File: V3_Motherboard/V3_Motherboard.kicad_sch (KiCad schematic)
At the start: 62 parts, among them J1 Conn_01x16_Pin, J10 Conn_02x04_Row_Letter_First, J14_GND2 Conn_01x03, J14_GND3 Conn_01x03, J18_VDC1 Conn_01x02, J2 Conn_01x16_Pin, J3 Conn_01x16_Pin, J4 Conn_01x16_Pin, J5 PINHD_1x2_Male, J6 Conn_01x02_Pin, J7 PINHD_1x2_Male, J8 PINHD_1x2_Male, J9 Conn_02x03_Counter_Clockwise, U1 NCV8164ASN250T1G_LDO_2.5V, U2 LTC4365TS8, U3 UM6K34NTCN

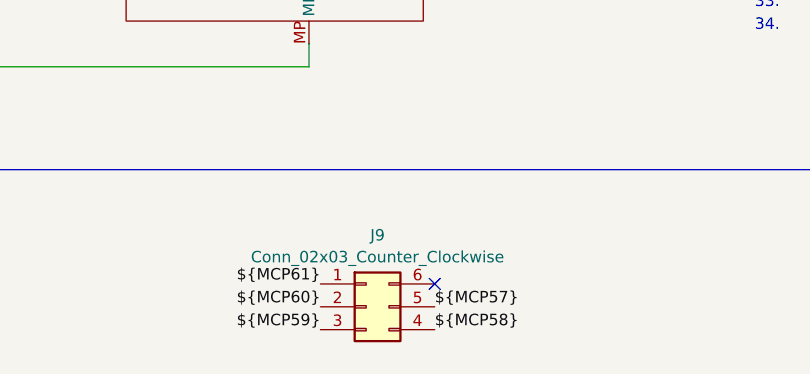
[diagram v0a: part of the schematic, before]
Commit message: Modded
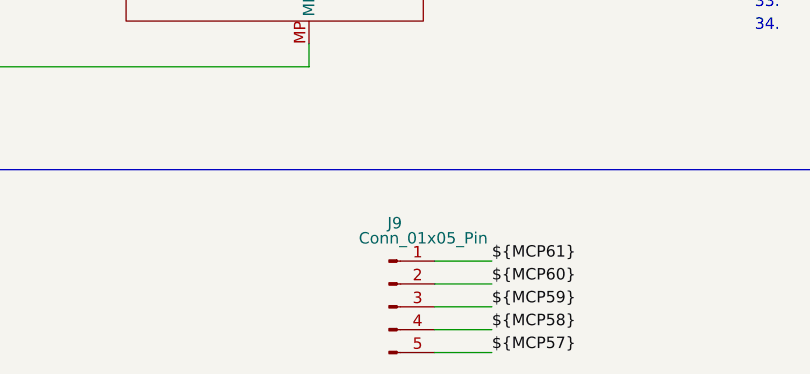
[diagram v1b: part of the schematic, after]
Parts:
- removed J9: Conn_02x03_Counter_Clockwise, Connector_PinHeader_2.54mm:PinHeader_2x03_P2.54mm_Vertical, symbol Connector_Generic:Conn_02x03_Counter_Clockwise
- added J9: Conn_01x05_Pin, Connector_PinHeader_2.54mm:PinHeader_1x05_P2.54mm_Vertical, symbol Connector:Conn_01x05_Pin
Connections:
- net ${MCP57}: now also J9.5 (Pin_5)
- net ${MCP58}: now also J9.4 (Pin_4)
- net ${MCP59}: now also J9.3 (Pin_3)
- net ${MCP60}: now also J9.2 (Pin_2)
- net ${MCP61}: now also J9.1 (Pin_1)
- no-connect marks 8 -> 7
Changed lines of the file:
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@@
 	)
 	(no_connect
-		(at 246.38 264.16)
-	)
-	(no_connect
 		(at 388.62 176.53)
 	)
@@
 	(wire
 		(pts
+			(xy 246.38 271.78) (xy 252.73 271.78)
+		)
+		(stroke
+			(width 0)
+			(type default)
+		)
+	)
+	(wire
+		(pts
 			(xy 318.77 36.83) (xy 316.23 36.83)
 		)
@@
 		)
 	)
+	(wire
+		(pts
+			(xy 246.38 269.24) (xy 252.73 269.24)
+		)
+		(stroke
+			(width 0)
+			(type default)
+		)
+	)
 	(polyline
 		(pts
@@
 	(wire
 		(pts
+			(xy 252.73 261.62) (xy 246.38 261.62)
+		)
+		(stroke
+			(width 0)
+			(type default)
+		)
+	)
+	(wire
+		(pts
 			(xy 317.5 39.37) (xy 328.93 39.37)
 		)
@@
 	(wire
 		(pts
+			(xy 252.73 266.7) (xy 246.38 266.7)
+		)
+		(stroke
+			(width 0)
+			(type default)
+		)
+	)
+	(wire
+		(pts
 			(xy 46.99 99.06) (xy 46.99 113.03)
 		)
@@
 		)
 	)
+	(wire
+		(pts
+			(xy 252.73 264.16) (xy 246.38 264.16)
+		)
+		(stroke
+			(width 0)
+			(type default)
+		)
+	)
 	(polyline
 		(pts
@@
 		)
 	)
-	(label "${MCP61}"
-		(at 233.68 264.16 180)
-		(effects
-			(font
-				(size 1.27 1.27)
-			)
-			(justify right bottom)
-		)
-	)
 	(label "${MCP16}"
 		(at 187.96 170.18 0)
@@
 		)
 	)
+	(label "${MCP59}"
+		(at 252.73 266.7 0)
+		(effects
+			(font
+				(size 1.27 1.27)
+			)
+			(justify left bottom)
+		)
+	)
+	(label "${MCP57}"
+		(at 252.73 271.78 0)
+		(effects
+			(font
+				(size 1.27 1.27)
+			)
+			(justify left bottom)
+		)
+	)
 	(label "${MCP46}"
 		(at 270.51 195.58 180)
@@
 		)
 	)
+	(label "${MCP58}"
+		(at 252.73 269.24 0)
+		(effects
+			(font
+				(size 1.27 1.27)
+			)
+			(justify left bottom)
+		)
+	)
 	(label "${MCP64}"
 		(at 186.69 223.52 0)
@@
 		)
 	)
-	(label "${MCP58}"
-		(at 246.38 269.24 0)
-		(effects
-			(font
-				(size 1.27 1.27)
-			)
-			(justify left bottom)
-		)
-	)
 	(label "${MCP53}"
 		(at 270.51 213.36 180)
@@
 		)
 	)
-	(label "${MCP59}"
-		(at 233.68 269.24 180)
-		(effects
-			(font
-				(size 1.27 1.27)
-			)
-			(justify right bottom)
-		)
-	)
 	(label "${MCP7}"
 		(at 187.96 193.04 0)
@@
 		)
 	)
-	(label "${MCP60}"
-		(at 233.68 266.7 180)
-		(effects
-			(font
-				(size 1.27 1.27)
-			)
-			(justify right bottom)
-		)
-	)
 	(label "VDD"
 		(at 191.77 144.78 180)
@@
 		)
 	)
-	(label "${MCP57}"
-		(at 246.38 266.7 0)
-		(effects
-			(font
-				(size 1.27 1.27)
-			)
-			(justify left bottom)
-		)
-	)
 	(label "${MCP52}"
 		(at 270.51 210.82 180)
@@
 		)
 	)
+	(label "${MCP60}"
+		(at 252.73 264.16 0)
+		(effects
+			(font
+				(size 1.27 1.27)
+			)
+			(justify left bottom)
+		)
+	)
 	(label "${MCP43}"
 		(at 115.57 177.8 0)
@@
 		)
 	)
+	(label "${MCP61}"
+		(at 252.73 261.62 0)
+		(effects
+			(font
+				(size 1.27 1.27)
+			)
+			(justify left bottom)
+		)
+	)
 	(label "${MCP5}"
 		(at 115.57 237.49 0)
@@
 	)
 	(symbol
-		(lib_id "Connector_Generic:Conn_02x03_Counter_Clockwise")
-		(at 238.76 266.7 0)
-		(unit 1)
-		(exclude_from_sim no)
-		(in_bom yes)
-		(on_board yes)
-		(dnp no)
-		(fields_autoplaced yes)
-		(property "Reference" "J9"
-			(at 240.03 258.7455 0)
-			(effects
-				(font
-					(size 1.27 1.27)
-				)
-			)
-		)
-		(property "Value" "Conn_02x03_Counter_Clockwise"
-			(at 240.03 261.1698 0)
-			(effects
-				(font
-					(size 1.27 1.27)
-				)
-			)
-		)
-		(property "Footprint" "Connector_PinHeader_2.54mm:PinHeader_2x03_P2.54mm_Vertical"
-			(at 238.76 266.7 0)
-			(effects
-				(font
-					(size 1.27 1.27)
-				)
-				(hide yes)
-			)
-		)
-		(property "Datasheet" "~"
-			(at 238.76 266.7 0)
-			(effects
-				(font
-					(size 1.27 1.27)
-				)
-				(hide yes)
-			)
-		)
-		(property "Description" "Generic connector, double row, 02x03, counter clockwise pin numbering scheme (similar to DIP package numbering), script generated (kicad-library-utils/schlib/autogen/connector/)"
-			(at 238.76 266.7 0)
-			(effects
-				(font
-					(size 1.27 1.27)
-				)
-				(hide yes)
-			)
-		)
-		(pin "5"
-		)
-		(pin "1"
-		)
-		(pin "3"
-		)
-		(pin "2"
-		)
-		(pin "6"
-		)
-		(pin "4"
-		)
-		(instances
-			(project ""
-				(path "/c83ca56d-bea6-42d1-99e0-b7b012709ff3"
-					(reference "J9")
-					(unit 1)
-				)
-			)
-		)
-	)
-	(symbol
 		(lib_id "Symbols-Library:LED")
 		(at 278.13 113.03 270)
@@
 					(unit 1)
 				)
+			)
+		)
+	)
+	(symbol
+		(lib_id "Connector:Conn_01x05_Pin")
+		(at 241.3 266.7 0)
+		(unit 1)
+		(exclude_from_sim no)
+		(in_bom yes)
+		(on_board yes)
+		(dnp no)
+		(property "Reference" "J9"
+			(at 241.935 257.3993 0)
+			(effects
+				(font
+					(size 1.27 1.27)
+				)
+			)
+		)
+		(property "Value" "Conn_01x05_Pin"
+			(at 245.11 259.08 0)
+			(effects
+				(font
+					(size 1.27 1.27)
+				)
+			)
+		)
+		(property "Footprint" "Connector_PinHeader_2.54mm:PinHeader_1x05_P2.54mm_Vertical"
+			(at 241.3 266.7 0)
+			(effects
+				(font
+					(size 1.27 1.27)
+				)
+				(hide yes)
+			)
+		)
+		(property "Datasheet" "~"
+			(at 241.3 266.7 0)
+			(effects
+				(font
+					(size 1.27 1.27)
+				)
+				(hide yes)
+			)
+		)
+		(property "Description" "Generic connector, single row, 01x05, script generated"
+			(at 241.3 266.7 0)
+			(effects
+				(font
+					(size 1.27 1.27)
+				)
+				(hide yes)
+			)
+		)
+		(pin "2"
+		)
+		(pin "3"
+		)
+		(pin "1"
+		)
+		(pin "4"
+		)
+		(pin "5"
+		)
+		(instances
+			(project ""
+				(path "/c83ca56d-bea6-42d1-99e0-b7b012709ff3"
+					(reference "J9")
+					(unit 1)
+				)

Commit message: Simplified PCB without LDO and additional breakouts
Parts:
- removed C4: 1u, Capacitor_SMD:C_0603_1608Metric, symbol Symbols-Library:C_Small
- removed C5: 10u, Capacitor_SMD:C_0603_1608Metric, symbol Symbols-Library:C_Small
- removed JP1_LDOPG1: Jumper_2_Open, Connector_PinHeader_2.54mm:PinHeader_1x02_P2.54mm_Vertical, symbol Symbols-Library:Jumper_2_Open
- removed R1, R3, R5: 1.1k, Resistor_SMD:R_0603_1608Metric, symbol Symbols-Library:R_1206
- removed R10: 10K, Resistor_SMD:R_0603_1608Metric, symbol Symbols-Library:R_1206
- removed R2, R4, R6: 3.3k, Resistor_SMD:R_0603_1608Metric, symbol Symbols-Library:R_1206
- removed U1: NCV8164ASN250T1G_LDO_2.5V, E6350_23:NCV8164ASN250T1G, symbol Symbols-Library:NCV8164ASN250T1G_LDO_2.5V
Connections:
- net CLK_CVRT_2.5V is gone; now on net CLK_CVRT_3.3V: J10.4 (Pin_4)
- net DATA_CVRT_2.5V is gone; now on net DATA_CVRT_3.3V: J10.2 (Pin_2)
- net EN_CVRT_2.5V is gone; now on net EN_CVRT_3.3V: J10.6 (Pin_6)
- net LDO_VIN is gone; now on net VIN: J18_VDC1.1 (Pin_1)
- net EN_MAN_2.5V renamed EN_MAN_3.3V
- net LDO_OUT_2.5V renamed VIN
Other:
- note added: "DIGITAL INPUT BREAKOUT"
- note added: "DIGITAL STATUS INDICATORS"
- note added: "VIN"
- note removed: "3.3V-2.5V LOGIC CONVERTERS"
- note removed: "CHIP 2.5V DIGITAL INPUTS"
- note removed: "LDO 2.5V OUTPUT"
- moved on the sheet: D2, D3, D4, R7, R8, R9
